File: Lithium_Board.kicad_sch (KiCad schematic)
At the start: 66 parts, among them IC1 BQ25750RRVR, IC2 TPS70933DBVR, J1 XT30PW-M, J2 XT30PW-F, J3 XT30PW-M, J5 TSW-105-07-G-S, Q1 SIR870ADP-T1-GE3, Q2 SIR870ADP-T1-GE3, Q3 SIR870ADP-T1-GE3, Q4 SIR870ADP-T1-GE3, Q5 SIR870ADP-T1-GE3, Q6 SIR870ADP-T1-GE3, Q7 SIR870ADP-T1-GE3, Q8 SIR870ADP-T1-GE3

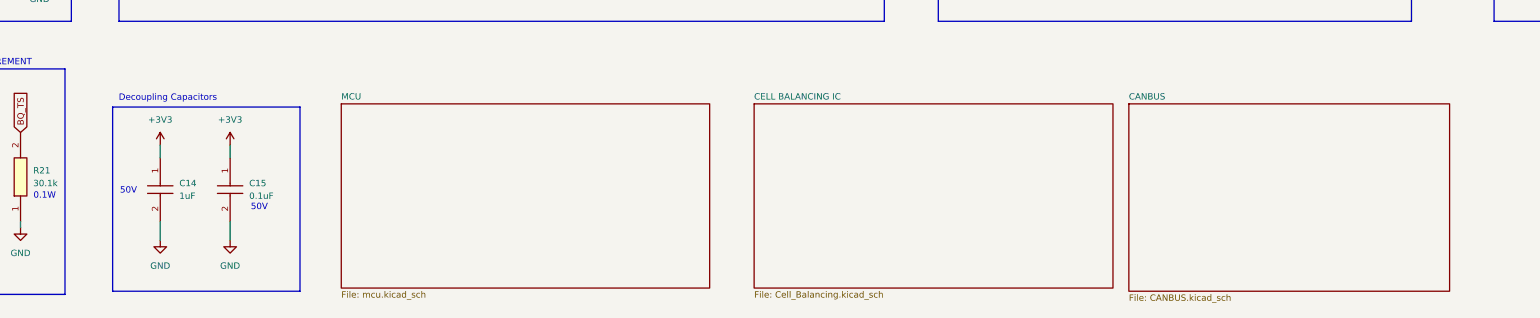
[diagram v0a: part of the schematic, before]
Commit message: First Layout Try
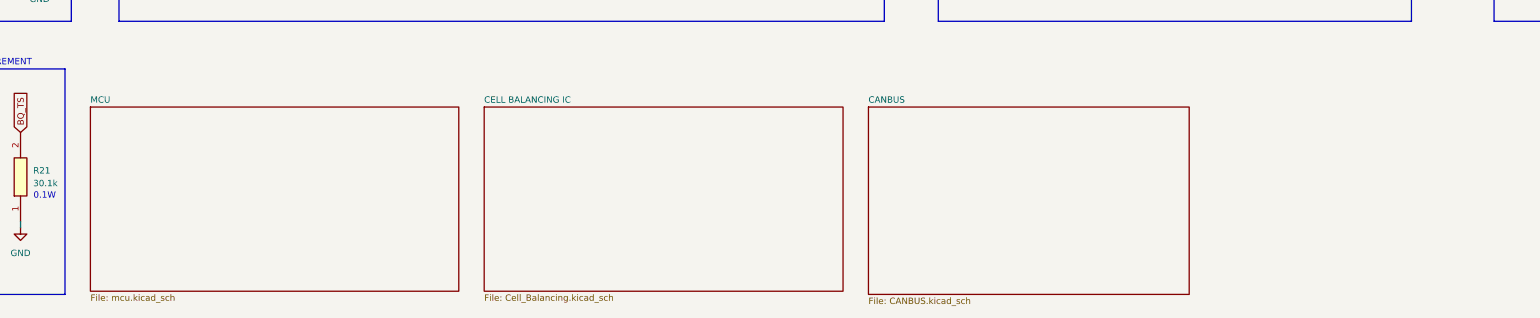
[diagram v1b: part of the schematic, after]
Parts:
- removed C14: 1uF, C2012X7R1H105K125AB:CAPC2012X145N, symbol C2012X7R1H105K125AB:C2012X7R1H105K125AB
- removed C15: 0.1uF, CC0603KRX7R9BB104:CAPC1608X90N, symbol CC0603KRX7R9BB104:CC0603KRX7R9BB104
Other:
- note removed: "Decoupling Capacitors"
